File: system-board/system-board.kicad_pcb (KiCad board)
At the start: 4 copper layers, 50 x 17.5 mm, 69 parts, among them IC1 Flash_16Mb, IC2 LSM6DSLTR, IC3 AP2115M-3.3TRG1, J1 BATT, J10 217183-0001, J2 GTFP08431BEU, J3 QWIIC, J4 SPKR, J5 BLADE_1, J6 BLADE_2, J7 BLADE_3, J8 BLADE_4, J9 BTNS, Q1 DMP1012UFDF, Q2 SSM6K504NU.LF, Q3 SSM6K504NU.LF, Q4 DMP1012UFDF, Q5 PMZB290UNE2YL, Q6 PMZB290UNE2YL, Q7 PMZB290UNE2YL, Q8 PMZB290UNE2YL, SW1 RST, SW2 USR, U1 MDBT50Q-1MV2, U2 MAX98357AETE+T, U3 BQ29705DSER, U4 MCP73832-2-OT, Y1 32.768k

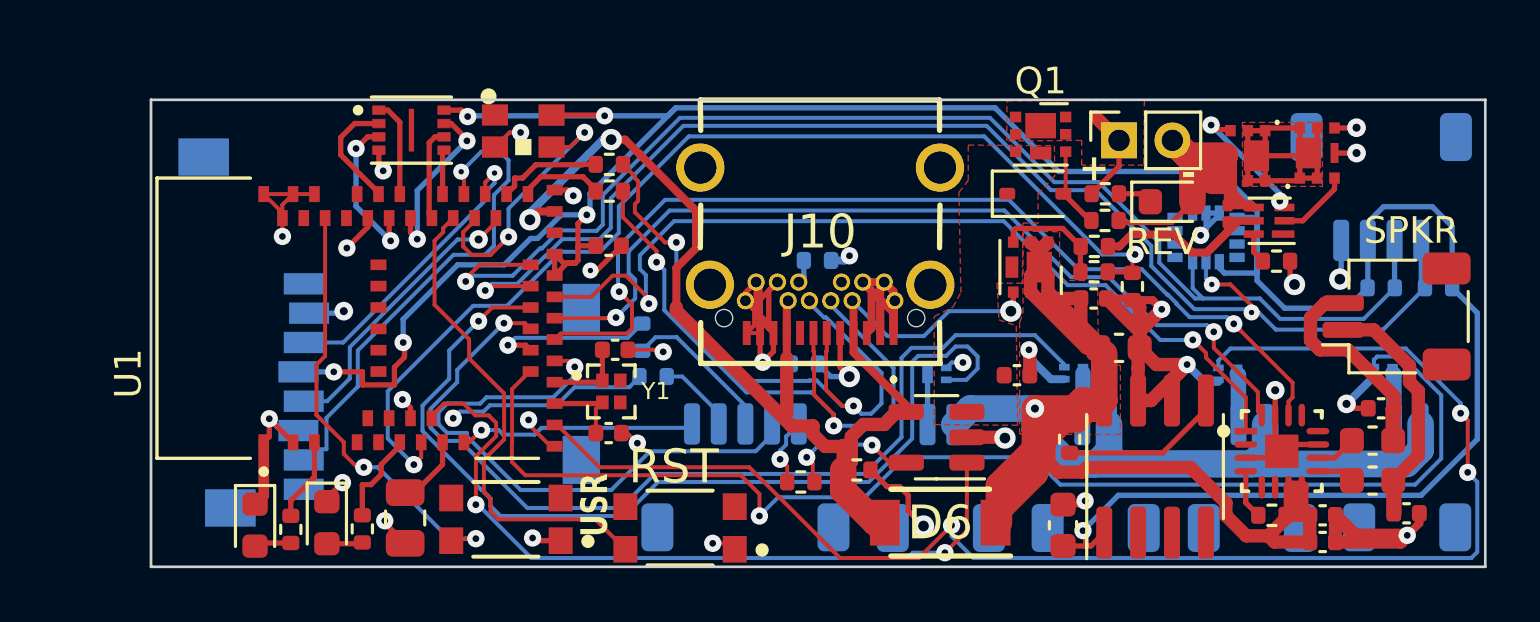
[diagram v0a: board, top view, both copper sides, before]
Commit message: First attempt
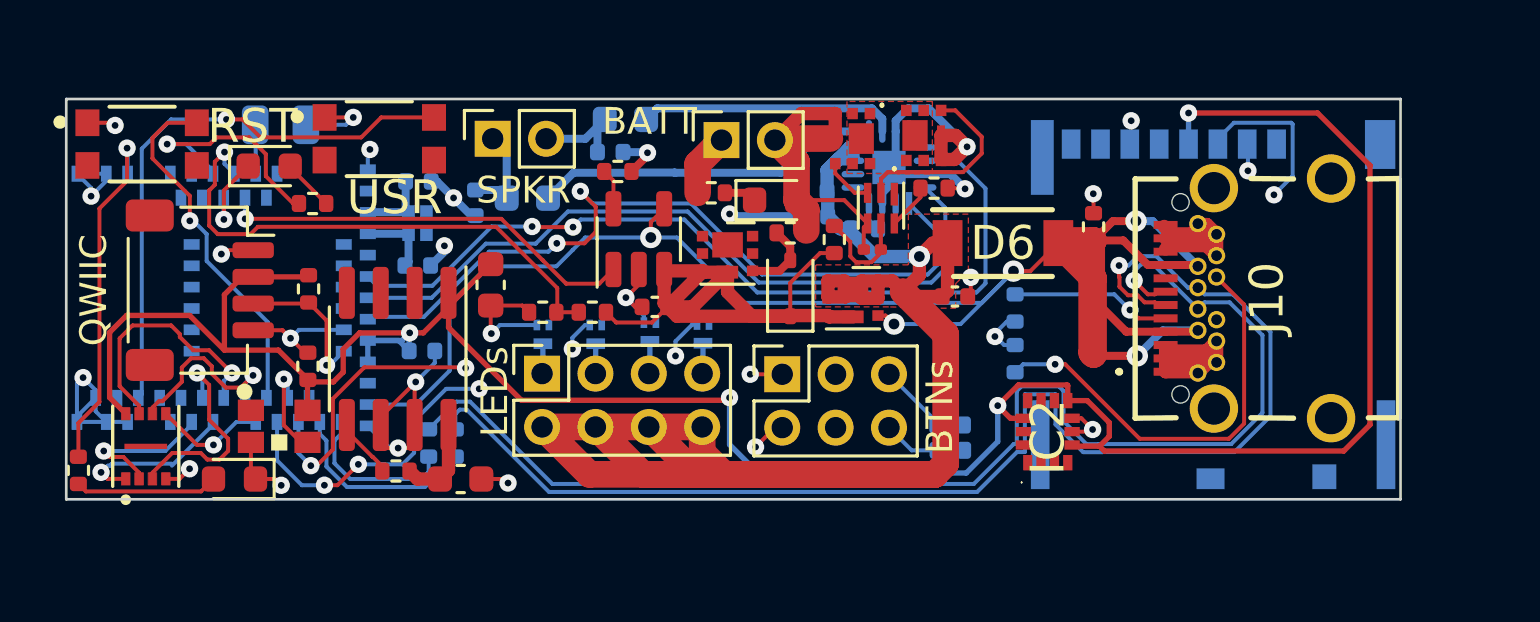
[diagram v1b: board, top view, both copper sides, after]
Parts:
- removed J5: BLADE_1, Connector_JST:JST_SH_SM02B-SRSS-TB_1x02-1MP_P1.00mm_Horizontal
- removed J6: BLADE_2, Connector_JST:JST_SH_SM02B-SRSS-TB_1x02-1MP_P1.00mm_Horizontal
- removed J7: BLADE_3, Connector_JST:JST_SH_SM02B-SRSS-TB_1x02-1MP_P1.00mm_Horizontal
- removed J8: BLADE_4, Connector_JST:JST_SH_SM02B-SRSS-TB_1x02-1MP_P1.00mm_Horizontal
- added J11: 503398-1892, Imports:Molex uSD Card Holder Push-Push 503398-1892, B.Cu at (116.8, 91.4)
- C1, C2, C3, C4, C5, C6, C7, C8, FB1, FB2, R1, R2, R7, U1, Y1: moved to B.Cu
- D1: value WS2812B -> WS2812B-2020
- IC2, J3, R5, R6: moved to F.Cu
- J2: value GTFP08431BEU -> LEDs; footprint Imports:GTFP08431BEU -> Connector_PinSocket_2.00mm:PinSocket_2x04_P2.00mm_Vertical; moved to F.Cu
- J4: footprint Connector_JST:JST_SH_SM02B-SRSS-TB_1x02-1MP_P1.00mm_Horizontal -> Connector_PinSocket_2.00mm:PinSocket_1x02_P2.00mm_Vertical
- J9: value BTNS -> BTNs; footprint Connector_JST:JST_SH_SM05B-SRSS-TB_1x05-1MP_P1.00mm_Horizontal -> Connector_PinSocket_2.00mm:PinSocket_2x03_P2.00mm_Vertical; moved to F.Cu
- U2: footprint MaximCustom:Maxim_Integrated-T1633-4-0-V-IPC_C -> Imports:Maxim_Integrated-T1633-4-0-V-IPC_C; moved to B.Cu
- moved J3 44.4 mm to (72.2, 98.2), turned to -90 degrees
- moved R6 42.5 mm to (76.3, 101.1), turned to -90 degrees
- moved R5 40.2 mm to (76.3, 98.2), turned to -90 degrees
- moved C6 36.8 mm to (82.6, 95.0), turned to 90 degrees
- moved J4 34.5 mm to (83.2, 92.6)
- moved FB2 33.4 mm to (84.5, 94.8), turned to 0 degrees
- moved Q5 31.5 mm to (85.1, 99.9), turned to -90 degrees
- moved FB1 30.5 mm to (88.2, 91.8), turned to 0 degrees
- moved C5 30.4 mm to (87.6, 93.1), turned to 180 degrees
- moved IC3 28.7 mm to (79.6, 100.8), turned to -90 degrees
- moved R15 25.3 mm to (79.6, 105.0), turned to 180 degrees
- moved C11 25.2 mm to (82.0, 105.3)
- moved SW1 24.8 mm to (70.1, 92.8), turned to 0 degrees
- moved Q6 23.7 mm to (87.1, 99.9), turned to -90 degrees
- moved C12 23.3 mm to (83.1, 98.0), turned to -90 degrees
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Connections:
- J2 pad 1: unconnected-(J2-DAT2-Pad1) -> /Blade LED Out/Blade_1_Out
- J2 pad 2: GND -> VDD
- J2 pad 3: /MOSI -> /Blade LED Out/Blade_2_Out
- J2 pad 4: VCC -> VDD
- J2 pad 5: /SCK -> /Blade LED Out/Blade_3_Out
- J2 pad 6: GND -> VDD
- J2 pad 7: /MISO -> /Blade LED Out/Blade_4_Out
- J2 pad 8: unconnected-(J2-DAT1-Pad8) -> VDD
- J9 pad 2: /A0 -> GND
- J9 pad 3: Net-(J9-Pin_3) -> /A0
- J9 pad 4: Net-(J9-Pin_4) -> /A2
- J9 pad 5: /A2 -> Net-(J9-Pin_5)
- R21 pad 1: Net-(J9-Pin_3) -> Net-(J9-Pin_5)
- R22 pad 1: Net-(J9-Pin_4) -> Net-(J9-Pin_6)
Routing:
- net /D10: track 54.1 -> 0.00 mm, vias 3 -> 0
- net /D9: track 47.4 -> 0.00 mm, vias 1 -> 0
- net /SCL: track 49.1 -> 4.41 mm, vias 3 -> 1
- net /SDA: track 48.1 -> 5.53 mm
- net /D6: track 36.1 -> 0.00 mm, vias 1 -> 0
- net /D5: track 35.7 -> 0.00 mm, vias 1 -> 0
- net /CONN_USB_D+: track 24.4 -> 50.0 mm, vias 2 -> 1
- net /CONN_USB_D-: track 24.6 -> 48.3 mm, vias 2 -> 1
- net /A0: track 21.7 -> 0.00 mm, vias 1 -> 0
- net /Power Management/BATT_PROT_+: track 4.20 -> 25.2 mm
- net /VDIV: track 40.1 -> 20.0 mm, vias 2 -> 1
- net /Power Management/VBUS: track 51.6 -> 69.6 mm, vias 3 -> 5
- net GND: track 107.9 -> 90.6 mm, vias 34 -> 30
- net Net-(J10-CC2): track 0.89 -> 16.0 mm, vias 0 -> 1
- net /A4: track 28.5 -> 15.6 mm, vias 2 -> 1
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- removed copper zone on F.Cu, net /Power Management/BATT_PROT_+
- removed copper zone on F.Cu, net /Power Management/BATT_RAW_+
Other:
- board size 50 x 17.5 mm -> 50 x 15 mm
- board text removed: "+"
- board text removed: "-"
